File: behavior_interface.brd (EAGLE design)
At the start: 83.7 x 141.5 mm, 44 parts, among them J8 POWER_JACK

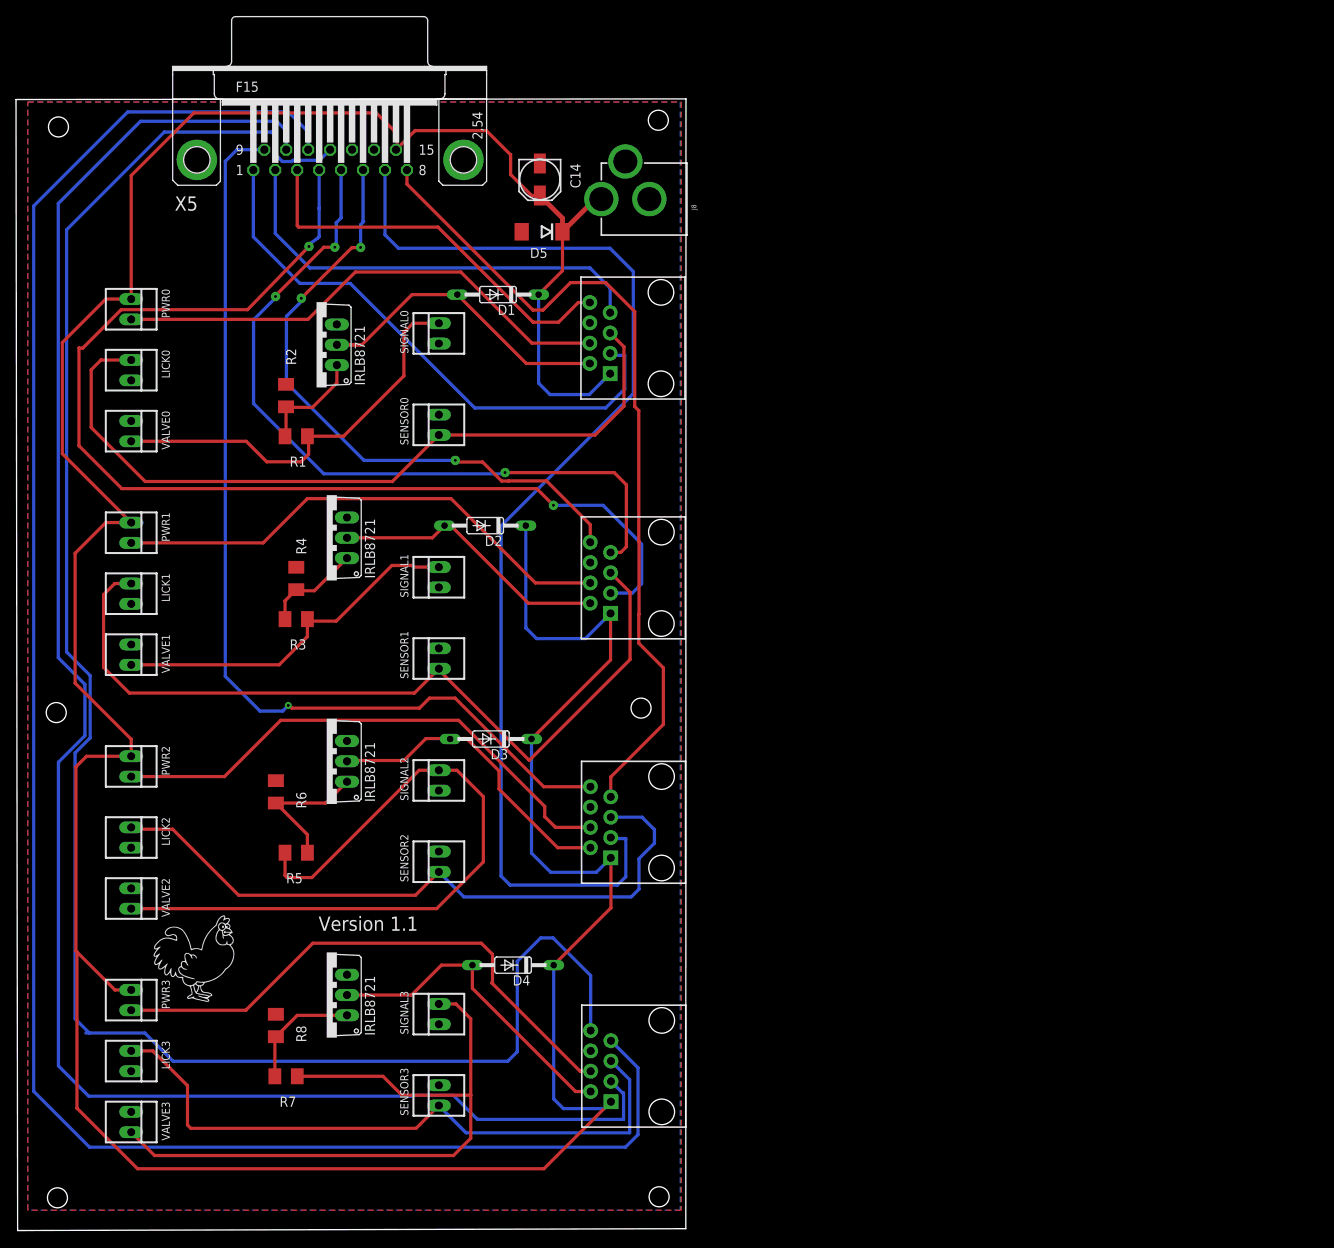
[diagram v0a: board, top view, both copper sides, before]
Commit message: update to latest version
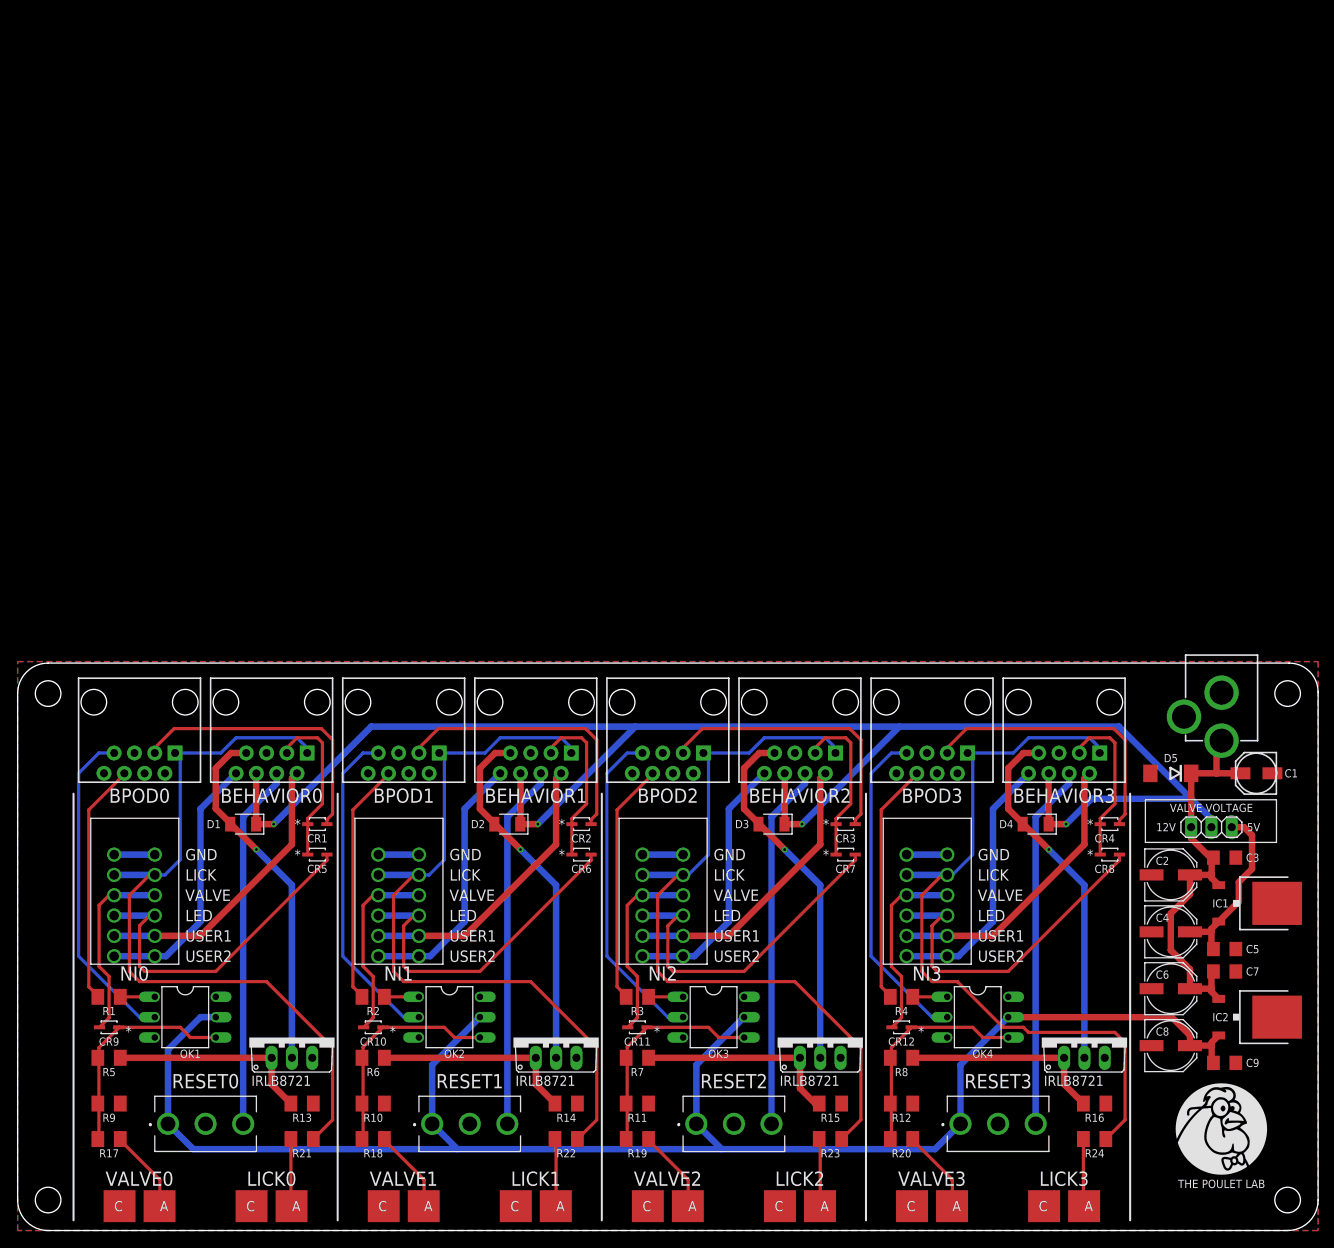
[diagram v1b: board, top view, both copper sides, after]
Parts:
- removed C14: EEE-FK1H100UR, JoshParts10:EEE-FK1H100UR
- removed PORT1, PORT2, PORT3, PORT4: RJ45-8PTH, SparkFun:RJ45-8
- removed PWR0, PWR1, PWR2, PWR3, SENSOR0, SENSOR1, SENSOR2, SENSOR3, SIGNAL0, SIGNAL1, SIGNAL2, SIGNAL3: 22-23-2021, con-molex:22-23-2021
- removed SETUP0: IRLB8721, IRLB8721:TO220V
- removed X5: (no value), con-subd:F15HP
- added BEHAVIOR0, BEHAVIOR1, BEHAVIOR2, BEHAVIOR3, BPOD0, BPOD1, BPOD2, BPOD3: RJ45-8PTH, SparkFun:RJ45-8
- added C1: EEE-FK1H100UR, JoshParts10:EEE-FK1H100UR
- added C2, C4, C6, C8: (no value), rcl:PANASONIC_D
- added C3, C5, C7, C9: (no value), rcl:C1206
- added CR1, CR10, CR11, CR12, CR2, CR3, CR4, CR5, CR6, CR7, CR8, CR9: CUS10S30USC_TOS-M, CUS10S30:USC_TOS-M
- added IC1, IC2: 7805DT, adafruit:TO252
- added JP1: (no value), pinhead:1X03
- added NI0, NI1, NI2, NI3: (no value), 1-2834015-6:1-2834015-6
- added OK1, OK2, OK3, OK4: CNY17, optocoupler:DIL06
- added R10, R11, R12, R13, R14, R15, R16, R9: 100k, rcl:M1206
- added R17, R18, R19, R20, R21, R22, R23, R24: 120, rcl:M1206
- added S1, S5, S6, S8: 734-6788, 734-6788:7346788
- added SETUP4: IRLB8721, IRLB8721:TO220V
- D1, D2, D3, D4: value 1N4148DO35-10 -> LL4148; device diode:DO35-10 -> Diode:DIOMELF3516
- LICK0, LICK1, LICK2, LICK3, VALVE0, VALVE1, VALVE2, VALVE3: value 22-23-2021 -> (none); device con-molex:22-23-2021 -> led:OSRAM-SIDELED
- R1, R3: value 1k -> 168
- R2, R4: value 100k -> 168
- R6, R8: value 100k -> 1k
- moved LICK3 118.0 mm to (130.8, 3.05)
- moved LICK0 106.0 mm to (31.8, 3.05)
- moved D5 103.7 mm to (144.1, 57.1)
- moved VALVE3 100.7 mm to (114.3, 3.05)
- moved VALVE0 96.9 mm to (15.2, 3.05)
- moved LICK2 95.4 mm to (97.8, 3.05)
- moved R4 92.0 mm to (110.5, 29.2), turned to 180 degrees
- moved LICK1 91.8 mm to (64.8, 3.05)
- moved J8 83.6 mm to (150.5, 74.9), turned to 180 degrees
- moved R8 78.3 mm to (110.5, 21.6), turned to 0 degrees
- moved VALVE2 77.3 mm to (81.3, 3.05)
- moved VALVE1 76.9 mm to (48.3, 3.05)
- moved R2 75.9 mm to (44.5, 29.2), turned to 180 degrees
- moved R1 73.9 mm to (11.4, 29.2)
- moved D1 73.5 mm to (28.2, 50.8)
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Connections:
- removed net 1: PORT1.3, X5.1
- removed net 10: PORT4.3, X5.10
- removed net 11: PORT4.7, X5.11
- removed net 12: PORT4.8, X5.12
- removed net 2: PORT1.7, X5.2
- removed net 3: PORT1.8, X5.3
- removed net 4: PORT2.3, X5.4
- removed net 5: PORT2.7, X5.5
- removed net 6: PORT2.8, X5.6
- removed net 7: PORT3.3, X5.7
- removed net 8: PORT3.7, X5.8
- removed net 9: PORT3.8, X5.9
- removed net N$17: PORT3.4, PWR2.2
- removed net N$45: X5.13
- removed net N$8: LICK1.1, PORT2.5, SENSOR1.1
- new net +12V: C1.ANODE, C2.+, C3.1, C6.+, C7.1, D5.C, IC1.1, IC2.1, J8.PWR, JP1.3
- new net +5V/2: BEHAVIOR0.6, BEHAVIOR1.6, BEHAVIOR2.6, BEHAVIOR3.6, D1.1, D2.1, D3.1, D4.1, JP1.2
- new net BPOD_VLVGND0: BPOD0.7, OK1.2
- new net BPOD_VLVGND1: BPOD1.7, OK2.2
- new net BPOD_VLVGND2: BPOD2.7, OK3.2
- new net BPOD_VLVGND3: BPOD3.7, OK4.2
- new net BPOD_VLVOUT0: BPOD0.6, R1.2
- new net BPOD_VLVOUT1: BPOD1.6, R2.2
- new net BPOD_VLVOUT2: BPOD2.6, R3.2
- new net BPOD_VLVOUT3: BPOD3.6, R4.2
- new net LED0: BEHAVIOR0.3, CR1.1, CR5.1
- new net LED1: BEHAVIOR1.3, CR2.1, CR6.1
- new net LED2: BEHAVIOR2.3, CR3.1, CR7.1
- new net LED3: BEHAVIOR3.3, CR4.1, CR8.1
- new net N$21: R15.2, R7.2, SETUP3.1
- new net N$22: BEHAVIOR2.7, D3.2, SETUP3.2
- new net N$23: BEHAVIOR2.4, S1.3
- new net N$24: OK3.1, R3.1
- new net N$25: BPOD2.3, CR3.2
- new net N$27: LICK2.A, R23.1
- new net N$28: R19.1, VALVE2.A
- new net N$29: C4.+, C5.1, IC1.2, JP1.1
- new net N$30: R16.2, R8.2, SETUP4.1
- new net N$32: BEHAVIOR3.7, D4.2, SETUP4.2
- new net N$35: BEHAVIOR3.4, S6.3
- new net N$36: OK4.1, R4.1
- new net N$37: BPOD3.3, CR4.2
- new net N$39: LICK3.A, R24.1
- new net N$40: R20.1, VALVE3.A
- new net NI_VALVE0: CR9.2, NI0.P$3, NI0.P$9
- new net NI_VALVE1: CR10.2, NI1.P$3, NI1.P$9
- new net NI_VALVE2: CR11.2, NI2.P$3, NI2.P$9
- new net NI_VALVE3: CR12.2, NI3.P$3, NI3.P$9
- new net SENSOR0: BEHAVIOR0.1, BPOD0.1, NI0.P$2, NI0.P$8, R21.2
- new net SENSOR1: BEHAVIOR1.1, BPOD1.1, NI1.P$2, NI1.P$8, R22.2
- new net SENSOR2: BEHAVIOR2.1, BPOD2.1, NI2.P$2, NI2.P$8, R23.2
- new net SENSOR3: BEHAVIOR3.1, BPOD3.1, NI3.P$2, NI3.P$8, R24.2
- new net USER1_0: BEHAVIOR0.2, NI0.P$11, NI0.P$5
- new net USER1_1: BEHAVIOR1.2, NI1.P$11, NI1.P$5
- new net USER1_2: BEHAVIOR2.2, NI2.P$11, NI2.P$5
- new net USER1_3: BEHAVIOR3.2, NI3.P$11, NI3.P$5
- new net USER2_0: BEHAVIOR0.8, NI0.P$12, NI0.P$6
- new net USER2_1: BEHAVIOR1.8, NI1.P$12, NI1.P$6
- new net USER2_2: BEHAVIOR2.8, NI2.P$12, NI2.P$6
- new net USER2_3: BEHAVIOR3.8, NI3.P$12, NI3.P$6
- new net VALVE0: CR9.1, OK1.4, R17.2, R5.1, R9.2
- new net VALVE1: CR10.1, OK2.4, R10.2, R18.2, R6.1
- new net VALVE2: CR11.1, OK3.4, R11.2, R19.2, R7.1
- new net VALVE3: CR12.1, OK4.4, R12.2, R20.2, R8.1
- net +5V: now also C8.+, C9.1, IC2.2, OK1.5, OK2.5, OK3.5, OK4.5, S1.1, S5.1, S6.1, S8.1; no longer C14.ANODE, D1.C, D2.C, D3.C, D4.C, D5.C, J8.PWR, PORT1.1, PORT2.1, PORT3.1, PORT4.1, PWR0.1, PWR1.1, PWR2.1, PWR3.1, X5.15
- net GND: now also BEHAVIOR0.5, BEHAVIOR1.5, BEHAVIOR2.5, BEHAVIOR3.5, BPOD0.5, BPOD1.5, BPOD2.5, BPOD3.5, C1.CATHODE, C2.-, C3.2, C4.-, C5.2, C6.-, C7.2, C8.-, C9.2, IC1.3, IC2.3, LICK0.C, LICK1.C, LICK2.C, LICK3.C, NI0.P$1, NI0.P$7, NI1.P$1, NI1.P$7, NI2.P$1, NI2.P$7, NI3.P$1, NI3.P$7, R10.1, R11.1, R12.1, R13.1, R14.1, R15.1, R16.1, R9.1, SETUP4.3, VALVE0.C, VALVE1.C, VALVE2.C, VALVE3.C; no longer C14.CATHODE, LICK0.2, LICK1.2, LICK2.2, LICK3.2, PORT1.6, PORT2.6, PORT3.6, PORT4.6, R2.1, R4.1, R6.1, R8.1, SENSOR0.2, SENSOR1.2, SENSOR2.2, SENSOR3.2, SETUP0.3, SIGNAL0.1, SIGNAL1.1, SIGNAL2.1, SIGNAL3.1, VALVE0.1, VALVE1.1, VALVE2.1, VALVE3.1, X5.14
- net N$1: now also R13.2, R5.2, SETUP1.1; no longer R1.1, SIGNAL0.2, VALVE0.2
- net N$10: now also LICK0.A, R21.1; no longer R5.2, R6.2, SETUP2.1
- net N$11: now also R17.1, VALVE0.A; no longer D3.A, PORT3.2, SETUP2.2
- net N$12: now also R14.2, R6.2, SETUP2.1; no longer LICK2.1, PORT3.5, SENSOR2.1
- net N$13: now also BEHAVIOR1.7, D2.2, SETUP2.2; no longer R7.1, SIGNAL3.2, VALVE3.2
- net N$14: now also BEHAVIOR1.4, S5.3; no longer R7.2, R8.2, SETUP3.1
- net N$15: now also OK2.1, R2.1; no longer D4.A, PORT4.2, SETUP3.2
- net N$16: now also BPOD1.3, CR2.2; no longer LICK3.1, PORT4.5, SENSOR3.1
- net N$18: now also CR7.2, NI2.P$10, NI2.P$4; no longer PORT1.4, PWR0.2
- net N$19: now also LICK1.A, R22.1; no longer PORT2.4, PWR1.2
- net N$2: now also CR5.2, NI0.P$10, NI0.P$4; no longer R1.2, R2.2, SETUP0.1
- net N$20: now also R18.1, VALVE1.A; no longer PORT4.4, PWR3.2
- net N$3: now also CR8.2, NI3.P$10, NI3.P$4; no longer D1.A, PORT1.2, SETUP0.2
- net N$4: now also BEHAVIOR0.7, D1.2, SETUP1.2; no longer LICK0.1, PORT1.5, SENSOR0.1
- net N$5: now also BEHAVIOR0.4, S8.3; no longer R3.1, SIGNAL1.2, VALVE1.2
- net N$6: now also OK1.1, R1.1; no longer R3.2, R4.2, SETUP1.1
- net N$7: now also BPOD0.3, CR1.2; no longer D2.A, PORT2.2, SETUP1.2
- net N$9: now also CR6.2, NI1.P$10, NI1.P$4; no longer R5.1, SIGNAL2.2, VALVE2.2
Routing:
- net 11: track 245.3 -> 0.00 mm
- net +5V: track 441.4 -> 206.5 mm
- net 12: track 231.0 -> 0.00 mm
- net 10: track 225.1 -> 0.00 mm
- net +5V/2: track 0.00 -> 213.7 mm, vias 0 -> 4
- net 7: track 146.6 -> 0.00 mm
- net 4: track 141.5 -> 0.00 mm, vias 2 -> 0
- net 9: track 122.9 -> 0.00 mm, vias 1 -> 0
- net 8: track 104.6 -> 0.00 mm
- net N$8: track 103.5 -> 0.00 mm
- net SENSOR1: track 0.00 -> 96.6 mm
- net SENSOR3: track 0.00 -> 96.6 mm
- net SENSOR0: track 0.00 -> 96.6 mm
- net SENSOR2: track 0.00 -> 96.3 mm
- net 5: track 95.6 -> 0.00 mm, vias 3 -> 0
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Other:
- board size 83.7 x 141.5 mm -> 162.6 x 70.9 mm
- board text added: "12V"
- board text added: "5V"
- board text added: "BEHAVIOR0"
- board text added: "BEHAVIOR1"
- board text added: "BEHAVIOR2"
- board text added: "BEHAVIOR3"
- board text added: "BPOD0"
- board text added: "BPOD1"
- board text added: "BPOD2"
- board text added: "BPOD3"
- board text added: "GND"
- board text added: "LED"
- board text added: "LICK"
- board text added: "RESET0"
- board text added: "RESET1"
- board text added: "RESET2"
- board text added: "RESET3"
- board text added: "THE POULET LAB"
- board text added: "USER1"
- board text added: "USER2"
- board text added: "VALVE"
- board text added: "VALVE VOLTAGE"
- board text removed: "D:/Dokumente/MDC/chicken1.bmp"
- board text removed: "Version 1.1"
